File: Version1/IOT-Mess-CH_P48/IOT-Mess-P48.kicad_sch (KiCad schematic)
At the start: 29 parts, among them J1 Conn_02x19_Odd_Even, J10 Jumper, J11 Jumper, J12 Jumper, J14 Jumper, J2 Conn_02x19_Odd_Even, J3 Jumper_2, J4 Jumper_2, J5 Conn_01x05_Pin, J6 Jumper, J7 Jumper, K1 Crystal, K32 Crystal, SW11 SW_Push, U10 USB_C_Receptacle_USB2.0_16P, U3 CH32L103C8T6, U6 ME6211C33M5

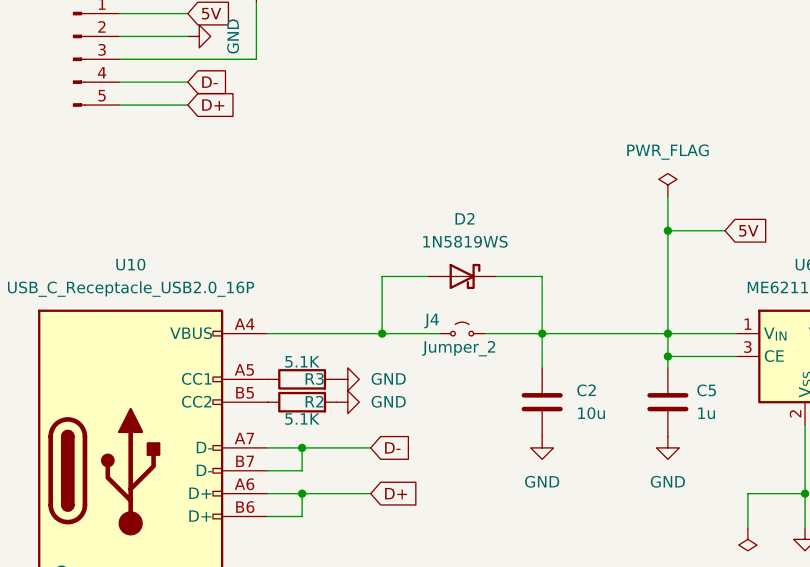
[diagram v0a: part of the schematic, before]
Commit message: updated.
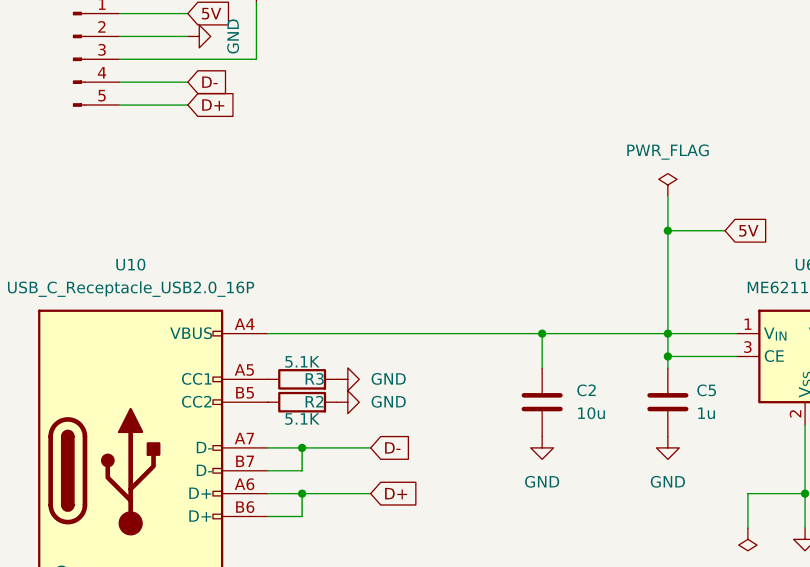
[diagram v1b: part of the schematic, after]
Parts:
- removed D2: 1N5819WS, Diode_SMD:D_SOD-323, symbol Diode:1N5819WS
- removed J4: Jumper_2, IOT-Mess-Footprints:Jumpper-triangle, symbol Jumper:Jumper_2_Small_Open
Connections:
- net 5V: now also U10.A4 (VBUS), U10.A9 (VBUS), U10.B4 (VBUS), U10.B9 (VBUS)
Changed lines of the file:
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@@
 	)
 	(junction
-		(at 86.36 217.17)
-		(diameter 0)
-		(color 0 0 0 0)
-	)
-	(junction
 		(at 133.35 234.95)
 		(diameter 0)
@@
 	(wire
 		(pts
-			(xy 104.14 210.82) (xy 104.14 217.17)
-		)
-		(stroke
-			(width 0)
-			(type default)
-		)
-	)
-	(wire
-		(pts
 			(xy 222.25 63.5) (xy 222.25 69.85)
 		)
@@
 	(wire
 		(pts
-			(xy 86.36 217.17) (xy 92.71 217.17)
-		)
-		(stroke
-			(width 0)
-			(type default)
-		)
-	)
-	(wire
-		(pts
 			(xy 118.11 201.93) (xy 118.11 205.74)
 		)
@@
 	(wire
 		(pts
-			(xy 86.36 210.82) (xy 91.44 210.82)
-		)
-		(stroke
-			(width 0)
-			(type default)
-		)
-	)
-	(wire
-		(pts
 			(xy 300.99 219.71) (xy 307.34 219.71)
 		)
@@
 	(wire
 		(pts
-			(xy 86.36 210.82) (xy 86.36 217.17)
-		)
-		(stroke
-			(width 0)
-			(type default)
-		)
-	)
-	(wire
-		(pts
 			(xy 104.14 220.98) (xy 104.14 217.17)
 		)
@@
 	(wire
 		(pts
-			(xy 99.06 210.82) (xy 104.14 210.82)
-		)
-		(stroke
-			(width 0)
-			(type default)
-		)
-	)
-	(wire
-		(pts
 			(xy 223.52 245.11) (xy 223.52 229.87)
 		)
@@
 	(wire
 		(pts
-			(xy 97.79 217.17) (xy 104.14 217.17)
-		)
-		(stroke
-			(width 0)
-			(type default)
-		)
-	)
-	(wire
-		(pts
 			(xy 77.47 232.41) (xy 77.47 229.87)
 		)
@@
 	(wire
 		(pts
-			(xy 73.66 217.17) (xy 86.36 217.17)
+			(xy 73.66 217.17) (xy 104.14 217.17)
 		)
 		(stroke
@@
 	)
 	(symbol
-		(lib_id "Jumper:Jumper_2_Small_Open")
-		(at 95.25 217.17 0)
-		(unit 1)
-		(exclude_from_sim no)
-		(in_bom yes)
-		(on_board yes)
-		(dnp no)
-		(property "Reference" "J4"
-			(at 91.948 215.646 0)
-			(effects
-				(font
-					(size 1.27 1.27)
-				)
-			)
-		)
-		(property "Value" "Jumper_2"
-			(at 94.996 218.694 0)
-			(effects
-				(font
-					(size 1.27 1.27)
-				)
-			)
-		)
-		(property "Footprint" "IOT-Mess-Footprints:Jumpper-triangle"
-			(at 95.25 217.17 0)
-			(effects
-				(font
-					(size 1.27 1.27)
-				)
-				(hide yes)
-			)
-		)
-		(property "Datasheet" "~"
-			(at 95.25 217.17 0)
-			(effects
-				(font
-					(size 1.27 1.27)
-				)
-				(hide yes)
-			)
-		)
-		(property "Description" "Jumper, 2-pole, small symbol, open"
-			(at 95.25 217.17 0)
-			(effects
-				(font
-					(size 1.27 1.27)
-				)
-				(hide yes)
-			)
-		)
-		(pin "1"
-		)
-		(pin "2"
-		)
-		(instances
-			(project "IOT-Mess-P48"
-				(path "/e8b1b29c-6130-44f1-99c5-074e206e80b8"
-					(reference "J4")
-					(unit 1)
-				)
-			)
-		)
-	)
-	(symbol
 		(lib_id "power:PWR_FLAG")
 		(at 118.11 201.93 0)
@@
 					(unit 1)
 				)
-			)
-		)
-	)
-	(symbol
-		(lib_id "Diode:1N5819WS")
-		(at 95.25 210.82 0)
-		(mirror y)
-		(unit 1)
-		(exclude_from_sim no)
-		(in_bom yes)
-		(on_board yes)
-		(dnp no)
-		(property "Reference" "D2"
-			(at 95.5675 204.47 0)
-			(effects
-				(font
-					(size 1.27 1.27)
-				)
-			)
-		)
-		(property "Value" "1N5819WS"
-			(at 95.5675 207.01 0)
-			(effects
-				(font
-					(size 1.27 1.27)
-				)
-			)
-		)
-		(property "Footprint" "Diode_SMD:D_SOD-323"
-			(at 95.25 215.265 0)
-			(effects
-				(font
-					(size 1.27 1.27)
-				)
-				(hide yes)
-			)
-		)
-		(property "Datasheet" "https://datasheet.lcsc.com/lcsc/2204281430_Guangdong-Hottech-1N5819WS_C191023.pdf"
-			(at 95.25 210.82 0)
-			(effects
-				(font
-					(size 1.27 1.27)
-				)
-				(hide yes)
-			)
-		)
-		(property "Description" "40V 600mV@1A 1A SOD-323 Schottky Barrier Diodes, SOD-323"
-			(at 95.25 210.82 0)
-			(effects
-				(font
-					(size 1.27 1.27)
-				)
-				(hide yes)
-			)
-		)
-		(pin "1"
-		)
-		(pin "2"
-		)
-		(instances
-			(project "IOT-Mess-P48"
-				(path "/e8b1b29c-6130-44f1-99c5-074e206e80b8"
-					(reference "D2")
-					(unit 1)
-				)
